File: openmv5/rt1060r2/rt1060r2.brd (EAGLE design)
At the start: 35.6 x 44.5 mm, 239 parts, among them CN1 S2B-PH-K-S(LF)(SN), IC1 LM66200DRLR, IC10 TCR2LF33,LM_CT, IC2 AP61300Z6-7, IC3 IS42S16160G-6BL, IC4 ATECC608B-MAHDA-T, IC5 IS25LP064D-JKLE-TR, IC7 MXC4005XC, IC8 MIMXRT1052DVL6B, IC9 KSZ8081RNDCA-TR, J1 USB4105-GF-A, J2 DNP, J3 DNP, J4 DF12-36-DS, J5 USD-1040310811, J6 DNP, J7 DNP, J8 3221-10-0300-00, M1 9774030151R, M2 9774030151R, Q1 2N7002KW_R1_00001, Q2 2N7002KW_R1_00001, Q3 2N7002KW_R1_00001, Q4 2N7002KW_R1_00001, Q5 2N7002KW_R1_00001, Q6 DMG2301L-7, Q7 2N7002KW_R1_00001, U2 BQ24075RGTR, U3 LBEE5KL1DX-883, Y1 SC32S-7PF20PPM, Y2 XRCGB24M000F3M00R0, Y3 ECS-327MVATX-3-CN-TR3

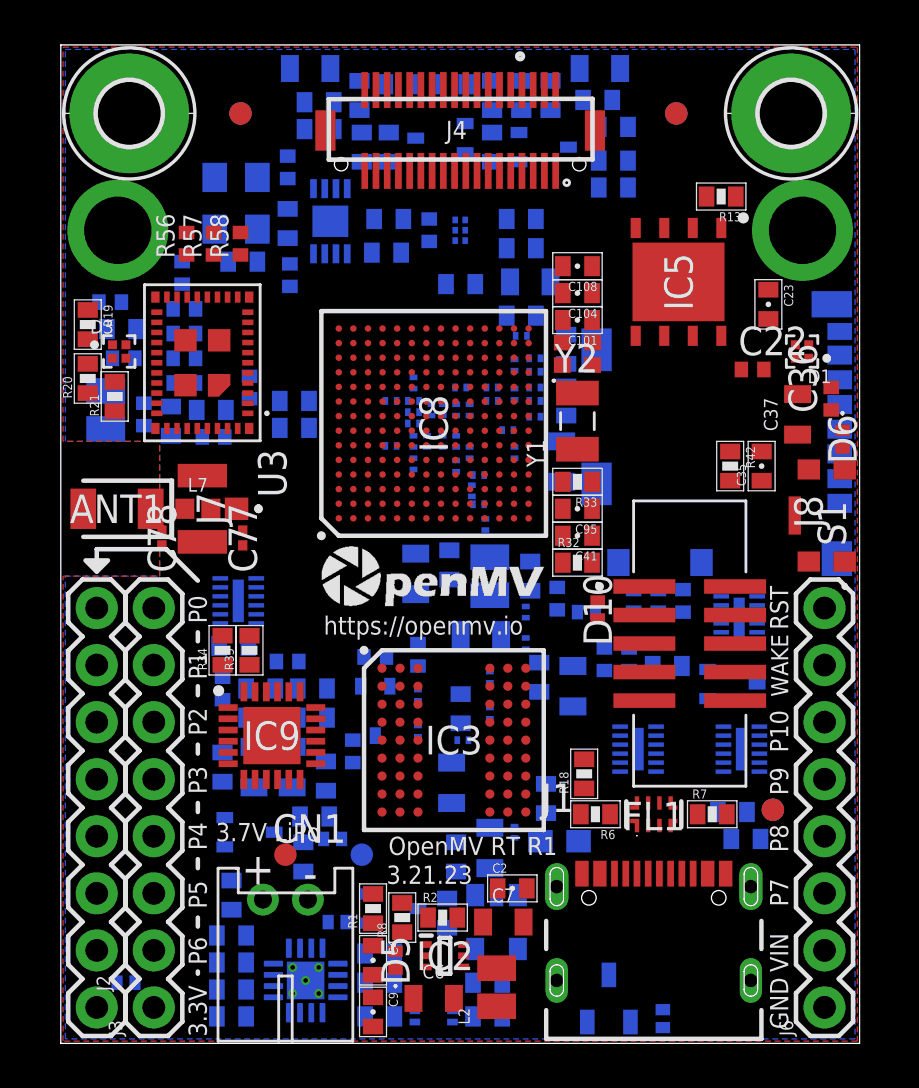
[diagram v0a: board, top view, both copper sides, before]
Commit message: Update R2 board per all feedback so far
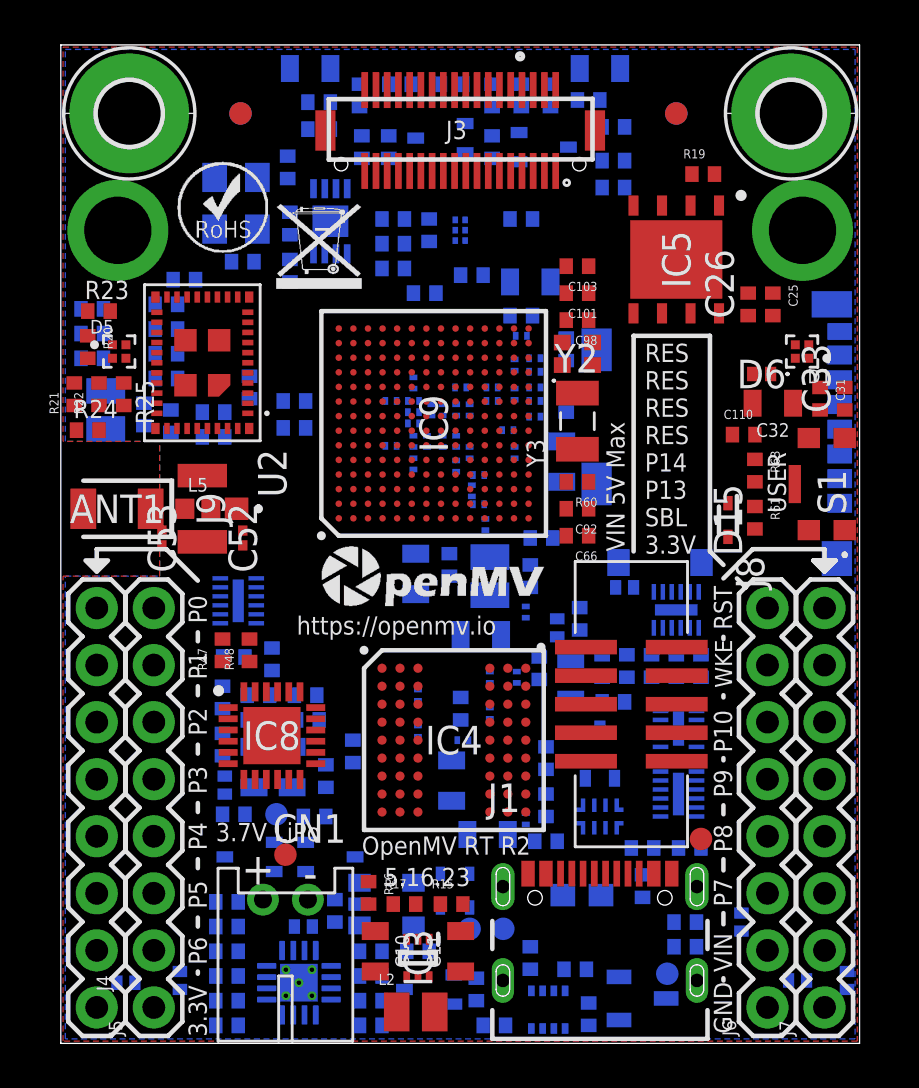
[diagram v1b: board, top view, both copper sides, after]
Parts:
- removed C111: 0.1uF, 0402:0402
- removed IC10: TCR2LF33,LM_CT, TCR2LF33_LM_CT:TCR2LF33LMCT
- removed L9: MAKK2016T2R2M, MAKK2016T2R2M:INDC2016X100N
- removed U3: LBEE5KL1DX-883, LBEE5KL1DX-TEMP:XCVR_LBEE5KL1DX-TEMP
- added C24: 0.22uF, rcl:C0201
- added C25: 4.7uF, 0402:0402
- added D11, D12, D13, D14: CPDQT5V0HE-HF, CPDQT5V0HE-HF:CPDQT5V0HEHF
- added D15: RB521S30T5G, RB521S30T5G:SODFL1608X70N
- added IC6: ATECC608B-MAHDA-T, ATECC608B-MAHDA-T:SON50P300X200X60-9N
- added J9: DNP, 2337019-1:23370191
- added L3: 100, 0402:0402
- added R60, R61, R63: 10K, 0402:0402
- added R62: 2.2M, 0402:0402
- added TP1, TP2: TPTP10R, testpad:TP10R
- added U1: BQ24075RGTR, BQ24075RGTR:QFN50P300X300X100-17N
- C1: value 4.7uF -> 1nF; device sfe:0402-CAP -> 0402:0402
- C10, C40, C65, C81: value 4.7uF -> 22uF; device sfe:0402-CAP -> SparkFun-Capacitors:0805
- C101, C2, C23, C27, C3, C35, C39, C4, C41, C42, C44, C5, C57, C72, C8, C9, C92: device sfe:0402-CAP -> 0402:0402
- C103, C13, C28, C31, C38, C43, C48, C59, C62, C66, C98: value 0.22uF -> 4.7uF; device rcl:C0201 -> 0402:0402
- C104, C12, C17, C21, C60, C64, C67, C83, C90, C91, C93, C95: value 4.7uF -> 0.22uF; device sfe:0402-CAP -> rcl:C0201
- C107: value 0.22uF -> 18pF
- C108: value 4.7uF -> 18pF; device sfe:0402-CAP -> rcl:C0201
- C11, C15, C19, C34, C45: value 0.22uF -> 22uF; device rcl:C0201 -> SparkFun-Capacitors:0805
- C110: value 1nF -> 4.7uF; device sfe:0402-CAP -> 0402:0402
- C14, C61, C73, C85, C96: value 22uF -> 0.22uF; device SparkFun-Capacitors:0805 -> rcl:C0201
- C18, C37, C58, C6, C7: value 22uF -> 4.7uF; device SparkFun-Capacitors:0805 -> 0402:0402
- C20: value 1uF -> 0.22uF; device 0402:0402 -> rcl:C0201
- C22, C74: value 0.1uF -> 22uF; device 0402:0402 -> SparkFun-Capacitors:0805
- C29: value 22uF -> 1uF; device SparkFun-Capacitors:0805 -> 0402:0402
- C30, C33, C46: value 4.7uF -> 0.1uF; device sfe:0402-CAP -> 0402:0402
- C36, C82, C84: value 0.1uF -> 4.7uF
- C47, C50, C54, C55, C56: value 0.22uF -> 0.1uF; device rcl:C0201 -> 0402:0402
- C51: value 22uF -> 0.1uF; device SparkFun-Capacitors:0805 -> 0402:0402
- C52: value 4.7uF -> GRM0335C1H1R5BA01D; device sfe:0402-CAP -> GRM0335C1H1R5BA01D:CAPC0603X33N
- C53: value 0.22uF -> DNP; device rcl:C0201 -> GRM0335C1H1R5BA01D:CAPC0603X33N
- C75, C76, C89: value 0.1uF -> 0.22uF; device 0402:0402 -> rcl:C0201
- C77: value GRM0335C1H1R5BA01D -> 4.7uF; device GRM0335C1H1R5BA01D:CAPC0603X33N -> 0402:0402
- C78: value DNP -> 22uF; device GRM0335C1H1R5BA01D:CAPC0603X33N -> SparkFun-Capacitors:0805
- C79: value 18pF -> 4.7uF; device rcl:C0201 -> 0402:0402
- C80: value 18pF -> 0.22uF
- D3: value UHD1110-FKA-CL1A13R3Q1BBQFMF3 -> RB521S30T5G; device UHD1110-FKA-CL1A13R3Q1BBQFMF3:LED_UHD1110-FKA-CL1A13R3Q1BBQFMF3 -> RB521S30T5G:SODFL1608X70N
- D4: value CPDQT5V0HE-HF -> RB521S30T5G; device CPDQT5V0HE-HF:CPDQT5V0HEHF -> RB521S30T5G:SODFL1608X70N
- D5: value CPDQT5V0HE-HF -> UHD1110-FKA-CL1A13R3Q1BBQFMF3; device CPDQT5V0HE-HF:CPDQT5V0HEHF -> UHD1110-FKA-CL1A13R3Q1BBQFMF3:LED_UHD1110-FKA-CL1A13R3Q1BBQFMF3
- IC2: value AP61300Z6-7 -> TCR2LF33,LM_CT; device AP61300Z6-7:SOTFL50P162X60-6N -> TCR2LF33_LM_CT:TCR2LF33LMCT
- IC3: value IS42S16160G-6BL -> AP61300Z6-7; device IS42S16160G-6BL:BGA54C80P9X9_800X800X120 -> AP61300Z6-7:SOTFL50P162X60-6N
- IC4: value ATECC608B-MAHDA-T -> IS42S16160G-6BL; device ATECC608B-MAHDA-T:SON50P300X200X60-9N -> IS42S16160G-6BL:BGA54C80P9X9_800X800X120
- IC5: value IS25LP064D-JKLE-TR -> IS25LP128F-JKLE-TR
- IC8: value MIMXRT1052DVL6B -> KSZ8081RNDCA-TR; device MIMXRT1052DVL6B:BGA196C65P14X14_1000X1000X143 -> KSZ8081RNDCA-TR:QFN50P400X400X90-25N
- IC9: value KSZ8081RNDCA-TR -> MIMXRT1052DVL6B; device KSZ8081RNDCA-TR:QFN50P400X400X90-25N -> MIMXRT1052DVL6B:BGA196C65P14X14_1000X1000X143
- J2: value DNP -> USD-1040310811; device SparkFun-Connectors:1X08 -> 1040310811:1040310811
- J3: value DNP -> DF12-36-DS; device SparkFun-Connectors:1X08 -> DF12-36-DS:DF12-36-DS
- J4: value DF12-36-DS -> DNP; device DF12-36-DS:DF12-36-DS -> SparkFun-Connectors:1X08
- J5: value USD-1040310811 -> DNP; device 1040310811:1040310811 -> SparkFun-Connectors:1X08
- J7: device 2337019-1:23370191 -> SparkFun-Connectors:1X08
- L4, L8: device sfe:C0402 -> 0402:0402
- L5: value MAKK2016T4R7M -> 3.9NH; device MAKK2016T4R7M:INDC2016X100N -> SparkFun-Coils:0402
- L6: value 100 -> MAKK2016T2R2M; device sfe:C0402 -> MAKK2016T2R2M:INDC2016X100N
- L7: value 3.9NH -> MAKK2016T4R7M; device SparkFun-Coils:0402 -> MAKK2016T4R7M:INDC2016X100N
- Q1: value 2N7002KW_R1_00001 -> DMG2301L-7; device 2N7002KW_R1_00001:SOT65P210X110-3N -> DMG2301L-7:SOT96P240X110-3N
- Q6: value DMG2301L-7 -> 2N7002KW_R1_00001; device DMG2301L-7:SOT96P240X110-3N -> 2N7002KW_R1_00001:SOT65P210X110-3N
- R1, R5: value 1K -> 5.1K; device sfe:0402-RES -> 0402:0402
- R10: value 1.1K -> 8.2K; device sfe:0402-RES -> 0402:0402
- R11: value 46.4K -> 100K; device sfe:0402-RES -> 0402:0402
- R12: value 8.2K -> 100K; device sfe:0402-RES -> 0402:0402
- R13, R18, R34, R36, R4: device sfe:0402-RES -> 0402:0402
- R15: value 2.7K -> 200K; device sfe:0402-RES -> 0402:0402
- R16: value 2.7K -> 100K; device sfe:0402-RES -> 0402:0402
- R17: value 2.7K -> 44.2K; device sfe:0402-RES -> 0402:0402
- R19, R35: value 220 -> 100K; device sfe:0402-RES -> 0402:0402
- R2: value 200K -> 5.1K; device sfe:0402-RES -> 0402:0402
- R20: value 220 -> 1K; device sfe:0402-RES -> 0402:0402
- R21: value 220 -> 10K; device sfe:0402-RES -> 0402:0402
- R22: value 100K -> 5.1K; device sfe:0402-RES -> 0402:0402
- R23, R24, R25: value 100K -> 10K; device sfe:0402-RES -> 0402:0402
- R26: value 1K -> 2.7K; device sfe:0402-RES -> 0402:0402
- R27: value 10K -> 2.7K; device sfe:0402-RES -> 0402:0402
- R28: value 100K -> 2.7K; device sfe:0402-RES -> 0402:0402
- R29, R33, R37: value 10K -> 100K; device sfe:0402-RES -> 0402:0402
- R3: value 100K -> 1M; device sfe:0402-RES -> 0402:0402
- R30, R31: value 4.7K -> 100K; device sfe:0402-RES -> 0402:0402
- R32: value 30K -> 100K; device sfe:0402-RES -> 0402:0402
- R38: value 6.49K -> 10K; device sfe:0402-RES -> 0402:0402
- R39: value 1K -> 100K; device sfe:0402-RES -> 0402:0402
- R40: value 2.2M -> 10K; device sfe:0402-RES -> 0402:0402
- R41: value 1M -> 4.7K; device sfe:0402-RES -> 0402:0402
- R42: value 10K -> 4.7K; device sfe:0402-RES -> 0402:0402
- R45, R46: value 100K -> DNP
- R48: value 100K -> 220
- R49, R51: value 100K -> 1K
- R50: value 100K -> 6.49K
- R52, R53: value 100K -> 10K
- R56, R57, R58: value 10K -> 100K
- R59: value 100K -> 30K
- R6, R7: value 5.1K -> 10K; device sfe:0402-RES -> 0402:0402
- R8: value 44.2K -> 1.1K; device sfe:0402-RES -> 0402:0402
- R9: value 10K -> 46.4K; device sfe:0402-RES -> 0402:0402
- U2: value BQ24075RGTR -> LBEE5KL1DX-883; device BQ24075RGTR:QFN50P300X300X100-17N -> LBEE5KL1DX-TEMP:XCVR_LBEE5KL1DX-TEMP
- Y1: value SC32S-7PF20PPM -> ECS-327MVATX-3-CN-TR3; device ABS07-32.768KHZ-7-T:XTAL_ABS07-32.768KHZ-7-T -> ECS-327MVATX-3-CN-TR3:ECS327MVATX3CNTR3
- Y3: value ECS-327MVATX-3-CN-TR3 -> SC32S-7PF20PPM; device ECS-327MVATX-3-CN-TR3:ECS327MVATX3CNTR3 -> ABS07-32.768KHZ-7-T:XTAL_ABS07-32.768KHZ-7-T
- moved J2 45.9 mm to (34.9, 33.1), flipped to the bottom, turned to 270 degrees
- moved J5 44.1 mm to (4.14, 1.60), flipped to the top, turned to 90 degrees
- moved J4 42.3 mm to (1.60, 1.60), turned to 90 degrees
- moved U$2 41.4 mm to (5.20, 35.2), flipped to the top
- moved J3 41.4 mm to (17.8, 40.6), turned to 0 degrees
- moved Q6 38.0 mm to (21.5, 39.9), turned to 180 degrees
- moved R41 36.9 mm to (11.5, 40.7)
- moved J7 35.5 mm to (34.0, 1.60)
- moved R46 35.4 mm to (28.0, 8.70)
- moved Q4 34.2 mm to (8.40, 8.30), turned to 0 degrees
- moved L4 33.2 mm to (7.20, 13.3), turned to 90 degrees
- moved Q5 32.4 mm to (12.0, 8.30), turned to 180 degrees
- moved R45 32.0 mm to (25.9, 7.00), turned to 90 degrees
- moved R38 31.0 mm to (24.6, 38.1)
- moved R15 30.7 mm to (17.4, 6.20), flipped to the top, turned to 0 degrees
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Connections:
- removed net SBL_BOOT: R42.2, S1.2, S1.3, S1.4
- new net JTAG_TDI_INT_UNUSED: J8.8, R45.2
- new net JTAG_TRSTB_INT_UNUSED: J8.9, R46.2
- new net PMIC_STBY_REQ: C110.2, D15.1, IC9.L7, R63.1
- new net SBL: D13.1, J6.2, R43.2
- new net SNVS_BAT: D4.2, TP1.TP
- new net SWITCH: D15.2, R61.1, R63.2, S1.2, S1.3, S1.4
- new net VDD_SNVS_CPU: C86.1, D3.1, D4.1, IC9.M9
- net ANT: now also C52.1, J9.1, L5.2, U2.41; no longer C77.1, J7.1, L7.2, U3.41
- net BAT: now also C5.2, U1.2, U1.3; no longer C8.2, U2.2, U2.3
- net BT_D_WAKE: now also IC9.L5, U2.39; no longer IC8.L5, U3.39
- net BT_H_WAKE: now also IC9.H14, R53.1, U2.38; no longer IC8.H14, R44.1, U3.38
- net BT_REG_ON: now also IC9.F13, R44.1, U2.14; no longer IC8.F13, R37.1, U3.14
- net BT_UART_CTS: now also IC9.L12, U2.5; no longer IC8.L12, U3.5
- net BT_UART_RTS: now also IC9.K12, U2.4; no longer IC8.K12, U3.4
- net BT_UART_RX: now also IC9.C9, U2.3; no longer IC8.C9, U3.3
- net BT_UART_TX: now also IC9.B9, U2.2; no longer IC8.B9, U3.2
- net CC1: now also R1.1; no longer R6.1
- net CC2: now also R2.1; no longer R7.1
- net CHG: now also R5.1, U1.9; no longer R1.1, U2.9
- net DCDC_LP: now also IC9.M1, IC9.M2, L7.2; no longer IC8.M1, IC8.M2, L5.2
- net DCDC_PSWITCH: now also C96.1, IC9.K3, R59.1; no longer C62.1, IC8.K3, R32.1
- net DCMI_CLK: now also IC9.B14, J3.12; no longer IC8.B14, J4.12
- net DCMI_D0: now also IC9.J14, J3.31; no longer IC8.J14, J4.31
- net DCMI_D1: now also IC9.G12, J3.29; no longer IC8.G12, J4.29
- net DCMI_D2: now also IC9.H11, J3.35; no longer IC8.H11, J4.35
- net DCMI_D3: now also IC9.H12, J3.28; no longer IC8.H12, J4.28
- net DCMI_D4: now also IC9.J13, J3.26; no longer IC8.J13, J4.26
- net DCMI_D5: now also IC9.L13, J3.33; no longer IC8.L13, J4.33
- net DCMI_D6: now also IC9.G14, J3.24; no longer IC8.G14, J4.24
- net DCMI_D7: now also IC9.F11, J3.22, R43.1; no longer IC8.F11, J4.22, S1.1, S1.5
- net DCMI_FSIN: now also J3.23, Q7.3, R39.1; no longer J4.23, Q5.3, R28.1
- net DCMI_HSYNC: now also IC9.L10, J3.18; no longer IC8.L10, J4.18
- net DCMI_MISO: now also IC9.E7, J3.15; no longer IC8.E7, J4.15
- net DCMI_MOSI: now also IC9.E8, J3.17; no longer IC8.E8, J4.17
- net DCMI_PCLK: now also IC9.D13, J3.14; no longer IC8.D13, J4.14
- net DCMI_PWDN: now also IC9.C11, J3.25, R40.1; no longer IC8.C11, J4.25, R29.1
- net DCMI_RST: now also IC9.B11, J3.21, R38.1; no longer IC8.B11, J4.21, R27.1
- net DCMI_SCL: now also IC9.J11, J3.32, R41.1; no longer IC8.J11, J4.32, R30.1
- net DCMI_SCLK: now also IC9.D8, J3.13; no longer IC8.D8, J4.13
- net DCMI_SDA: now also IC9.K11, J3.34, R42.1; no longer IC8.K11, J4.34, R31.1
- net DCMI_SSEL: now also IC9.D7, J3.11, R37.1; no longer IC8.D7, J4.11, R24.1
- net DCMI_VSYNC: now also IC9.D14, J3.16; no longer IC8.D14, J4.16
- net EN: now also IC3.5, Q5.3, R16.1; no longer IC2.5, Q1.3, R3.1
- net ETH_INT: now also IC8.18, IC9.C10, R49.1; no longer IC8.C10, IC9.18, R36.1
- net ETH_LED: now also IC8.23, R48.1; no longer IC9.23, R35.1
- net ETH_MDC: now also IC8.11, IC9.A7; no longer IC8.A7, IC9.11
- net ETH_MDIO: now also IC8.10, IC9.C7, R51.1; no longer IC8.C7, IC9.10, R39.1
- net ETH_RST: now also C42.2, IC8.24, IC9.D10, R47.1; no longer C65.2, IC8.D10, IC9.24, R34.1
- net ETH_RXD0: now also IC8.13, IC9.E12; no longer IC8.E12, IC9.13
- net ETH_RXD1: now also IC8.12, IC9.D12; no longer IC8.D12, IC9.12
- net ETH_RXDV: now also IC8.15, IC9.C12; no longer IC8.C12, IC9.15
- net ETH_RXERR: now also IC8.17, IC9.C13; no longer IC8.C13, IC9.17
- net ETH_TXCLK: now also IC8.8, IC9.B13; no longer IC8.B13, IC9.8
- net ETH_TXD0: now also IC8.20, IC9.B12; no longer IC8.B12, IC9.20
- net ETH_TXD1: now also IC8.21, IC9.A12; no longer IC8.A12, IC9.21
- net ETH_TXEN: now also IC8.19, IC9.A13; no longer IC8.A13, IC9.19
- net ETH_VDDA_3.3: now also C43.2, C45.1, C46.1, IC8.2, L4.1; no longer C81.2, C82.1, C85.1, IC9.2, L8.1
- net ETH_VDD_1.2: now also C44.2, C47.1, IC8.1; no longer C83.2, C84.1, IC9.1
- net FB: now also IC3.1, R15.1, R17.2; no longer IC2.1, R2.1, R8.2
- net FEED: now also C53.1, L5.1; no longer C78.1, L7.1
- net GND: now also C10.2, C104.2, C108.2, C11.2, C12.1, C17.2, C19.1, C21.2, C23.2, C24.1, C25.1, C28.1, C33.2, C36.1, C37.1, C38.1, C40.2, C43.1, C46.2, C48.1, C49.2, C52.2, C59.1, C6.1, C60.2, C61.2, C62.1, C68.2, C7.1, C73.2, C74.1, C77.1, C78.1, C79.1, C85.1, C86.2, C87.2, C88.1, C89.1, C90.2, C99.2, D11.2, D12.2, D13.2, D14.2, IC3.2, IC4.A1, IC4.A3, IC4.B7, IC4.C3, IC4.D7, IC4.E3, IC4.J1, IC6.4, IC6.9, IC8.22, IC8.25, IC9.A1, IC9.A14, IC9.B10, IC9.B5, IC9.E13, IC9.E2, IC9.G7, IC9.G8, IC9.H7, IC9.H8, IC9.J7, IC9.J8, IC9.K13, IC9.K2, IC9.K6, IC9.K9, IC9.L9, IC9.N1, IC9.N2, IC9.N5, IC9.N8, IC9.P1, IC9.P14, J2.CD$2, J2.G$1, J2.G$2, J2.G$3, J2.G$4, J2.P$6, J3.19, J3.27, J3.5, J5.1, J7.1, J9.2, J9.3, Q1.1, R1.2, R17.1, R2.2, R3.2, R44.2, R50.2, R62.2, R8.2, S1.1, S1.5, TP2.TP, U1.15, U1.17, U1.4, U1.6, U1.8, U2.1, U2.12, U2.19, U2.21, U2.29, U2.32, U2.33, U2.35, U2.40, U2.42, U2.43, U2.44, U2.45, U2.46, Y1.2; no longer C10.1, C104.1, C108.1, C11.1, C111.2, C12.2, C17.1, C19.2, C21.1, C23.1, C28.2, C33.1, C36.2, C37.2, C38.2, C40.1, C43.2, C46.1, C48.2, C49.1, C52.1, C59.2, C6.2, C60.1, C61.1, C62.2, C68.1, C7.2, C73.1, C74.2, C77.2, C78.2, C79.2, C85.2, C86.1, C87.1, C88.2, C89.2, C90.1, C99.1, D4.2, D5.2, IC10.2, IC3.A1, IC3.A3, IC3.B7, IC3.C3, IC3.D7, IC3.E3, IC3.J1, IC4.4, IC4.9, IC8.A1, IC8.A14, IC8.B10, IC8.B5, IC8.E13, IC8.E2, IC8.G7, IC8.G8, IC8.H7, IC8.H8, IC8.J7, IC8.J8, IC8.K13, IC8.K2, IC8.K6, IC8.K9, IC8.L9, IC8.N1, IC8.N2, IC8.N5, IC8.N8, IC8.P1, IC8.P14, IC9.22, IC9.25, J3.1, J4.19, J4.27, J4.5, J5.CD$2, J5.G$1, J5.G$2, J5.G$3, J5.G$4, J5.P$6, J6.1, J7.2, J7.3, Q6.1, R11.2, R12.2, R27.2, R37.2, R40.2, R41.2, R6.2, R8.1, U2.15, U2.17, U2.4, U2.6, U2.8, U3.1, U3.12, U3.19, U3.21, U3.29, U3.32, U3.33, U3.35, U3.40, U3.42, U3.43, U3.44, U3.45, U3.46, Y3.2
- net ILIM: now also R8.1, U1.12; no longer R10.1, U2.12
- net INT_I2C_INT: now also IC9.D11, R28.1; no longer IC8.D11, R17.1
- net INT_I2C_SCL: now also IC6.6, IC9.C8, R26.1; no longer IC4.6, IC8.C8, R15.1
- net INT_I2C_SDA: now also IC6.5, IC9.B8, R27.1; no longer IC4.5, IC8.B8, R16.1
- net ISET: now also R10.1, U1.16; no longer R12.1, U2.16
- net JTAG_TCK: now also FL5.5, IC9.F12; no longer FL5.4, IC8.F12
- net JTAG_TCK_INT: now also FL5.8; no longer FL5.9
- net JTAG_TDI: now also FL5.3, IC9.F14; no longer FL5.2, IC8.F14
- net JTAG_TDI_INT: now also FL5.10, J6.4, R45.1; no longer FL5.11, J8.8
- net JTAG_TDO: now also FL5.4, IC9.G13; no longer FL5.3, IC8.G13
- net JTAG_TDO_INT: now also FL5.9; no longer FL5.10
- net JTAG_TMS: now also FL5.6, IC9.E14; no longer FL5.5, IC8.E14
- net JTAG_TMS_INT: now also FL5.7; no longer FL5.8
- net JTAG_TRSTB: now also FL5.1, IC9.G10; no longer FL5.6, IC8.G10
- net JTAG_TRSTB_INT: now also FL5.12, J6.3, R46.1; no longer FL5.7, J8.9
- net LED_B: now also IC9.C14, R20.1, R23.1; no longer IC8.C14, R19.1, R56.1
- net LED_B_INT: now also D5.1, R20.2; no longer D3.1, R19.2
- net LED_CHG: now also R5.2; no longer R1.2
- net LED_G: now also IC9.A10, R21.1, R24.1; no longer IC8.A10, R20.1, R57.1
- net LED_G_INT: now also D5.2, R21.2; no longer D3.2, R20.2
- net LED_PGOOD: now also R6.2; no longer R4.2
- net LED_R: now also IC9.D9, R22.1, R25.1; no longer IC8.D9, R21.1, R58.1
- net LED_R_INT: now also D5.3, R22.2; no longer D3.3, R21.2
- net LED_ST: now also R4.2; no longer R5.2
- net LPO_IN: now also U2.37, Y1.3; no longer U3.37, Y3.3
- net MDI_LED: now also J5.8, R48.2; no longer J3.8, R35.2
- net MDI_RX_N: now also IC8.3, J5.7; no longer IC9.3, J3.7
- net MDI_RX_P: now also IC8.4, J5.6; no longer IC9.4, J3.6
- net MDI_TX_N: now also IC8.5, J5.5; no longer IC9.5, J3.5
- net MDI_TX_P: now also IC8.6, J5.4; no longer IC9.6, J3.4
- net NVCC_PLL: now also C101.2, C102.1, IC9.P10; no longer C104.2, C107.1, IC8.P10
- net ONOFF: now also IC9.M6, Q4.2; no longer IC8.M6, Q3.2
- net ON_BATTERY: now also IC9.P2, Q2.2, R12.1; no longer IC8.P2, Q7.2, R59.1
- net P0_MOSI: now also FL3.1, IC9.H10; no longer FL2.1, IC8.H10
- net P0_MOSI_INT: now also FL3.12, J4.8; no longer FL2.12, J2.8
- net P10_PWM: now also Q6.3, R36.1; no longer Q4.3, R26.1
- net P10_PWM_INT: now also J7.6; no longer J6.6
- net P11_WAKEUP: now also Q3.3, R13.1; no longer Q2.3, R22.1
- net P11_WAKEUP_INT: now also J7.7; no longer J6.7
- net P12_RST_N: now also C109.1, FL5.2, IC9.M7, R60.2; no longer C63.1, FL5.1, IC8.M7, R33.2
- net P12_RST_N_EXT: now also FL5.11, J7.8; no longer FL5.12, J6.8
- net P1_MISO: now also FL3.2, IC9.M11; no longer FL2.2, IC8.M11
- net P1_MISO_INT: now also FL3.11, J4.7; no longer FL2.11, J2.7
- net P2_SCLK: now also FL3.3, IC9.M14; no longer FL2.3, IC8.M14
- net P2_SCLK_INT: now also FL3.10, J4.6; no longer FL2.10, J2.6
- net P3_NSS: now also FL3.4, IC9.G11; no longer FL2.4, IC8.G11
- net P3_NSS_INT: now also FL3.9, J4.5; no longer FL2.9, J2.5
- net P4_SCL: now also FL3.5, IC9.K14; no longer FL2.5, IC8.K14
- net P4_SCL_INT: now also FL3.8, J4.4; no longer FL2.8, J2.4
- net P5_SDA: now also FL3.6, IC9.L14; no longer FL2.6, IC8.L14
- net P5_SDA_INT: now also FL3.7, J4.3; no longer FL2.7, J2.3
- net P6_ADC: now also IC9.M12; no longer IC8.M12
- net P6_ADC_INT: now also J4.2; no longer J2.2
- net P7_PWM: now also IC9.A8; no longer IC8.A8
- net P7_PWM_INT: now also J7.3; no longer J6.3
- net P8_PWM: now also IC9.A9; no longer IC8.A9
- net P8_PWM_INT: now also J7.4; no longer J6.4
- net P9_PWM: now also IC9.A11; no longer IC8.A11
- net P9_PWM_INT: now also J7.5; no longer J6.5
- net PGOOD: now also Q2.3, R11.1, R6.1, U1.7; no longer Q7.3, R14.1, R4.1, U2.7
- net PMIC_ONOFF: now also D11.1, J5.3, Q4.3, R14.1; no longer D8.1, J3.3, Q3.3, R23.1
- net PMIC_ON_REQ: now also IC9.K7, Q5.2; no longer IC8.K7, Q1.2
- net PWM_FSIN: now also IC9.M5, Q6.2, Q7.2, R35.1; no longer IC8.M5, Q4.2, Q5.2, R25.1
- net P_FLASH_CE: now also IC9.L3, R19.2; no longer IC8.L3, R13.2
- net P_FLASH_IO0: now also IC9.P3; no longer IC8.P3
- net P_FLASH_IO1: now also IC9.N4; no longer IC8.N4
- net P_FLASH_IO2: now also IC9.P4; no longer IC8.P4
- net P_FLASH_IO3: now also IC9.P5; no longer IC8.P5
- net P_FLASH_SCK: now also IC9.L4; no longer IC8.L4
- net RAW: now also C10.1, C7.2, C8.2, D9.1, IC2.1, IC3.3, J5.2, R11.2, R13.2, R16.2, U1.10, U1.11, U1.5; no longer C1.2, C10.2, C6.1, D5.1, IC10.1, IC10.3, J3.2, R22.2, R23.2, R3.2, U2.10, U2.11, U2.5
- net REXT: now also IC8.9, R50.1; no longer IC9.9, R38.1
- net RTC_XTALI: now also C108.1, IC9.N9, Y3.2; no longer C80.1, IC8.N9, Y1.2
- net RTC_XTALO: now also C107.1, IC9.P9, Y3.1; no longer C79.1, IC8.P9, Y1.1
- net SDRAM_A0: now also IC4.H7, IC9.C2; no longer IC3.H7, IC8.C2
- net SDRAM_A1: now also IC4.H8, IC9.G1; no longer IC3.H8, IC8.G1
- net SDRAM_A10: now also IC4.H9, IC9.G2; no longer IC3.H9, IC8.G2
- net SDRAM_A11: now also IC4.G2, IC9.B4; no longer IC3.G2, IC8.B4
- net SDRAM_A12: now also IC4.G1, IC9.A3; no longer IC3.G1, IC8.A3
- net SDRAM_A2: now also IC4.J8, IC9.G3; no longer IC3.J8, IC8.G3
- net SDRAM_A3: now also IC4.J7, IC9.H1; no longer IC3.J7, IC8.H1
- net SDRAM_A4: now also IC4.J3, IC9.A6; no longer IC3.J3, IC8.A6
- net SDRAM_A5: now also IC4.J2, IC9.B6; no longer IC3.J2, IC8.B6
- net SDRAM_A6: now also IC4.H3, IC9.B1; no longer IC3.H3, IC8.B1
- net SDRAM_A7: now also IC4.H2, IC9.A5; no longer IC3.H2, IC8.A5
- net SDRAM_A8: now also IC4.H1, IC9.A4; no longer IC3.H1, IC8.A4
- net SDRAM_A9: now also IC4.G3, IC9.B2; no longer IC3.G3, IC8.B2
- net SDRAM_BA0: now also IC4.G7, IC9.C1; no longer IC3.G7, IC8.C1
- net SDRAM_BA1: now also IC4.G8, IC9.F1; no longer IC3.G8, IC8.F1
- net SDRAM_CAS: now also IC4.F7, IC9.D3; no longer IC3.F7, IC8.D3
- net SDRAM_CKE: now also IC4.F3, IC9.A2; no longer IC3.F3, IC8.A2
- net SDRAM_CLK: now also IC4.F2, IC9.B3; no longer IC3.F2, IC8.B3
- net SDRAM_CS: now also IC4.G9, IC9.E1; no longer IC3.G9, IC8.E1
- net SDRAM_DQ0: now also IC4.A8, IC9.E3; no longer IC3.A8, IC8.E3
- net SDRAM_DQ1: now also IC4.B9, IC9.F3; no longer IC3.B9, IC8.F3
- net SDRAM_DQ10: now also IC4.D1, IC9.D5; no longer IC3.D1, IC8.D5
- net SDRAM_DQ11: now also IC4.C2, IC9.C4; no longer IC3.C2, IC8.C4
- net SDRAM_DQ12: now also IC4.C1, IC9.D4; no longer IC3.C1, IC8.D4
- net SDRAM_DQ13: now also IC4.B2, IC9.E5; no longer IC3.B2, IC8.E5
- net SDRAM_DQ14: now also IC4.B1, IC9.C3; no longer IC3.B1, IC8.C3
- net SDRAM_DQ15: now also IC4.A2, IC9.E4; no longer IC3.A2, IC8.E4
- net SDRAM_DQ2: now also IC4.B8, IC9.F4; no longer IC3.B8, IC8.F4
- net SDRAM_DQ3: now also IC4.C9, IC9.G4; no longer IC3.C9, IC8.G4
- net SDRAM_DQ4: now also IC4.C8, IC9.F2; no longer IC3.C8, IC8.F2
- net SDRAM_DQ5: now also IC4.D9, IC9.G5; no longer IC3.D9, IC8.G5
- net SDRAM_DQ6: now also IC4.D8, IC9.H5; no longer IC3.D8, IC8.H5
- net SDRAM_DQ7: now also IC4.E9, IC9.H4; no longer IC3.E9, IC8.H4
- net SDRAM_DQ8: now also IC4.E1, IC9.C6; no longer IC3.E1, IC8.C6
- net SDRAM_DQ9: now also IC4.D2, IC9.C5; no longer IC3.D2, IC8.C5
- net SDRAM_DQMH: now also IC4.F1, IC9.D6; no longer IC3.F1, IC8.D6
- net SDRAM_DQML: now also IC4.E8, IC9.H3; no longer IC3.E8, IC8.H3
- net SDRAM_RAS: now also IC4.F8, IC9.D2; no longer IC3.F8, IC8.D2
- net SDRAM_WE: now also IC4.F9, IC9.D1; no longer IC3.F9, IC8.D1
- net SD_CD: now also D7.1, IC9.L11, J2.CD$1, R29.1; no longer D9.1, IC8.L11, J5.CD$1, R50.1
- net SD_CLK: now also FL2.4, IC9.J3; no longer FL3.4, IC8.J3
- net SD_CLK_INT: now also FL2.9, J2.P$5; no longer FL3.9, J5.P$5
- net SD_CMD: now also FL2.3, IC9.J4, R32.1; no longer FL3.3, IC8.J4, R53.1
- net SD_CMD_INT: now also FL2.10, J2.P$3; no longer FL3.10, J5.P$3
- net SD_DAT0: now also FL2.5, IC9.J1, R31.1; no longer FL3.5, IC8.J1, R52.1
- net SD_DAT0_INT: now also FL2.8, J2.P$7; no longer FL3.8, J5.P$7
- net SD_DAT1: now also FL2.6, IC9.K1, R30.1; no longer FL3.6, IC8.K1, R51.1
- net SD_DAT1_INT: now also FL2.7, J2.P$8; no longer FL3.7, J5.P$8
- net SD_DAT2: now also FL2.1, IC9.H2, R34.1; no longer FL3.1, IC8.H2, R55.1
- net SD_DAT2_INT: now also FL2.12, J2.P$1; no longer FL3.12, J5.P$1
- net SD_DAT3: now also FL2.2, IC9.J2, R33.1; no longer FL3.2, IC8.J2, R54.1
- net SD_DAT3_INT: now also FL2.11, J2.P$2; no longer FL3.11, J5.P$2
- net SHELL_GND: now also C1.2, R3.1; no longer C110.2, R41.1
- net SR_VLX: now also L6.1, U2.34; no longer L9.1, U3.34
- net ST: now also R4.1; no longer R5.1
- net SW: now also IC3.4; no longer IC2.4
- net TMR: now also R9.1, U1.14; no longer R11.1, U2.14
- net TS: now also R7.1, U1.1; no longer R9.1, U2.1
- net USB_D_N: now also IC9.M8; no longer IC8.M8
- net USB_D_P: now also IC9.L8; no longer IC8.L8
- net VBUS: now also C2.2, C90.1, C92.2, IC9.N6; no longer C3.2, C88.1, C95.2, IC8.N6
- net VCC: now also C103.2, C104.1, C11.1, C12.2, C17.1, C19.2, C21.1, C23.1, C24.2, C25.2, C28.2, C33.1, C34.1, C36.2, C37.2, C38.2, C48.2, C49.1, C51.1, C59.2, C69.1, C70.1, C71.1, C77.2, C78.2, C82.1, C83.2, C84.1, C85.2, C88.2, C95.2, D12.1, D14.1, D5.4, D8.1, IC3.6, IC4.A7, IC4.A9, IC4.B3, IC4.C7, IC4.D3, IC4.E7, IC4.J9, IC6.8, IC8.14, IC9.E6, IC9.E9, IC9.F10, IC9.F5, IC9.J10, IC9.J6, IC9.K4, IC9.K5, IC9.L1, IC9.L2, IC9.P12, J2.P$4, J3.10, J3.2, J3.20, J3.30, J3.36, J4.1, J6.1, L3.2, Q2.1, Q6.1, R12.2, R19.1, R23.2, R27.2, R33.2, R35.2, R37.2, R40.2, R41.2, R42.2, R60.1, U2.30, U2.36, Y1.1, Y1.4; no longer C108.2, C109.1, C11.2, C111.1, C12.1, C17.2, C19.1, C21.2, C23.2, C28.1, C33.2, C36.1, C37.1, C40.2, C41.2, C42.2, C43.1, C44.2, C53.1, C54.1, C57.2, C64.1, C68.2, C7.1, C86.2, C89.1, C90.2, C92.2, C93.2, C96.1, C99.2, D10.1, D3.4, D4.1, IC2.6, IC3.A7, IC3.A9, IC3.B3, IC3.C7, IC3.D3, IC3.E7, IC3.J9, IC4.8, IC8.E6, IC8.E9, IC8.F10, IC8.F5, IC8.J10, IC8.J6, IC8.K4, IC8.K5, IC8.L1, IC8.L2, IC8.P12, IC9.14, J2.1, J4.10, J4.2, J4.20, J4.30, J4.36, J5.P$4, L6.2, Q4.1, Q5.1, R13.1, R16.2, R17.2, R2.2, R33.1, R42.1, R43.2, R44.2, R45.2, R46.2, R48.2, R50.2, U3.30, U3.36, Y3.1, Y3.4
- net VCC_SOC: now also C60.1, C61.1, C62.2, C63.1, C64.1, C65.2, C68.1, C89.2, C91.2, C93.2, IC9.F6, IC9.F7, IC9.F8, IC9.F9, IC9.G6, IC9.G9, IC9.H6, IC9.H9, IC9.J5, IC9.J9, L7.1; no longer C103.2, C34.1, C38.1, C45.1, C46.2, C47.1, C48.1, C49.2, C87.2, C98.2, IC8.F6, IC8.F7, IC8.F8, IC8.F9, IC8.G6, IC8.G9, IC8.H6, IC8.H9, IC8.J5, IC8.J9, L5.1
- net VDDA: now also C40.1, C41.2, J3.4, L3.1; no longer C51.1, C52.2, J4.4, L4.1
- net VDDA_ADC_3P3: now also C72.2, C73.1, C74.2, IC9.N14, L8.1; no longer C59.1, C60.2, C61.2, IC8.N14, L6.1
- net VDD_HIGH_CAP: now also C98.2, C99.1, IC9.P8; no longer C101.2, C102.1, IC8.P8
- net VDD_SNVS: now also C9.2, D3.2, IC2.5, Q4.1, Q5.1, R61.2; no longer C2.2, C69.1, IC10.5, IC8.M9, Q1.1, Q2.1
- net VDD_SNVS_CAP: now also C87.1, IC9.M10; no longer C70.1, IC8.M10
- net VDD_USB_CAP: now also C79.2, C80.1, C81.2, IC9.K8; no longer C71.1, C72.2, C73.2, IC8.K8
- net VIN: now also D10.1, J7.2, Q1.3; no longer D7.1, J6.2, Q6.3
- net VIN_INT: now also C4.2, Q1.2; no longer C5.2, Q6.2
- net VIN_LDO: now also C54.1, C57.2, L6.2, U2.31; no longer C74.1, C91.2, L9.2, U3.31
- net V_BATT: now also C3.2, C6.2, U1.13; no longer C4.2, C9.2, U2.13
- net WAKEUP: now also IC9.L6, Q3.2; no longer IC8.L6, Q2.2
- net WIFI_CLK: now also IC9.M13, U2.20; no longer IC8.M13, U3.20
- net WIFI_CMD: now also IC9.H13, R58.1, U2.22; no longer IC8.H13, R49.1, U3.22
- net WIFI_D0: now also IC9.M4, R57.1, U2.24; no longer IC8.M4, R48.1, U3.24
- net WIFI_D1: now also IC9.M3, R56.1, U2.26; no longer IC8.M3, R47.1, U3.26
- net WIFI_D2: now also IC9.J12, R55.1, U2.23; no longer IC8.J12, R46.1, U3.23
- net WIFI_D3: now also IC9.K10, R54.1, U2.25; no longer IC8.K10, R45.1, U3.25
- net WL_H_WAKE: now also IC9.E11, R52.1, U2.27; no longer IC8.E11, R43.1, U3.27
- net WL_REG_ON: now also IC9.E10, U2.28; no longer IC8.E10, U3.28
- net XTALI: now also IC9.P11, R62.1; no longer IC8.P11, R40.1
- net XTALO: now also IC9.N11; no longer IC8.N11
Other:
- board text added: "5.16.23"
- board text added: "OpenMV RT R2"
- board text added: "RES RES RES RES P14 P13 SBL 3.3V"
- board text added: "USER"
- board text added: "WKE"
- board text removed: "3.21.23"
- board text removed: "IR"
- board text removed: "OpenMV RT R1"
- board text removed: "W"
- board text removed: "WAKE"
